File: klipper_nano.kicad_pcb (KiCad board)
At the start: 2 copper layers, 59.8 x 88.9 mm, 54 parts, among them J1 UART1, J10 ACC_PWR, J11 ACC_SPI, J2 PWR_IN, J3 TFT, J4 USB_A, J5 USB_A, J6 PWR_OUT, J7 USB_B_Mini, J8 UART2, J9 PWC, Q1 IRLML6344TRPBF, Q2 IRLML6402, U1 FT230XS, U2 PC817, U3 74HC04, U4 74HC4094, U5 74HC4094, U6 74HC4040, U7 ISO7721, U8 USBLC6-4SC6

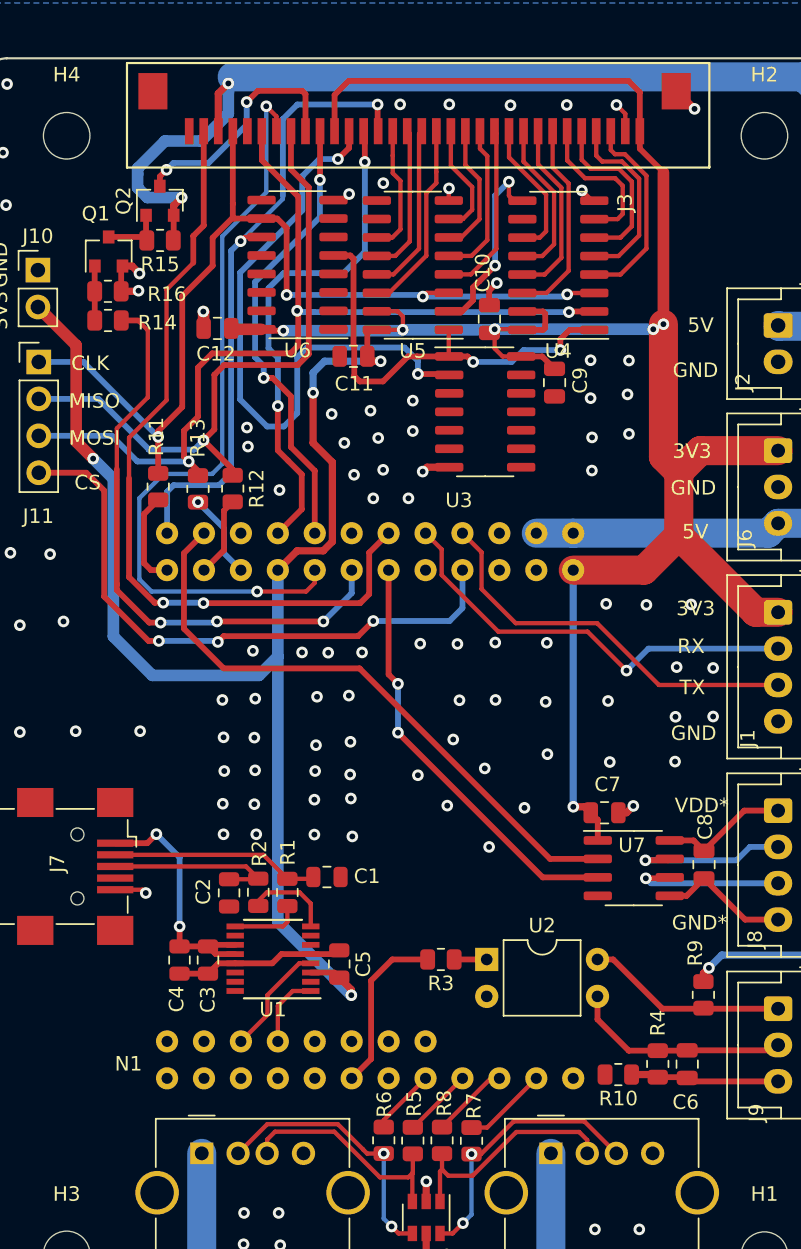
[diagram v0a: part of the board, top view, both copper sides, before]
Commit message: v2
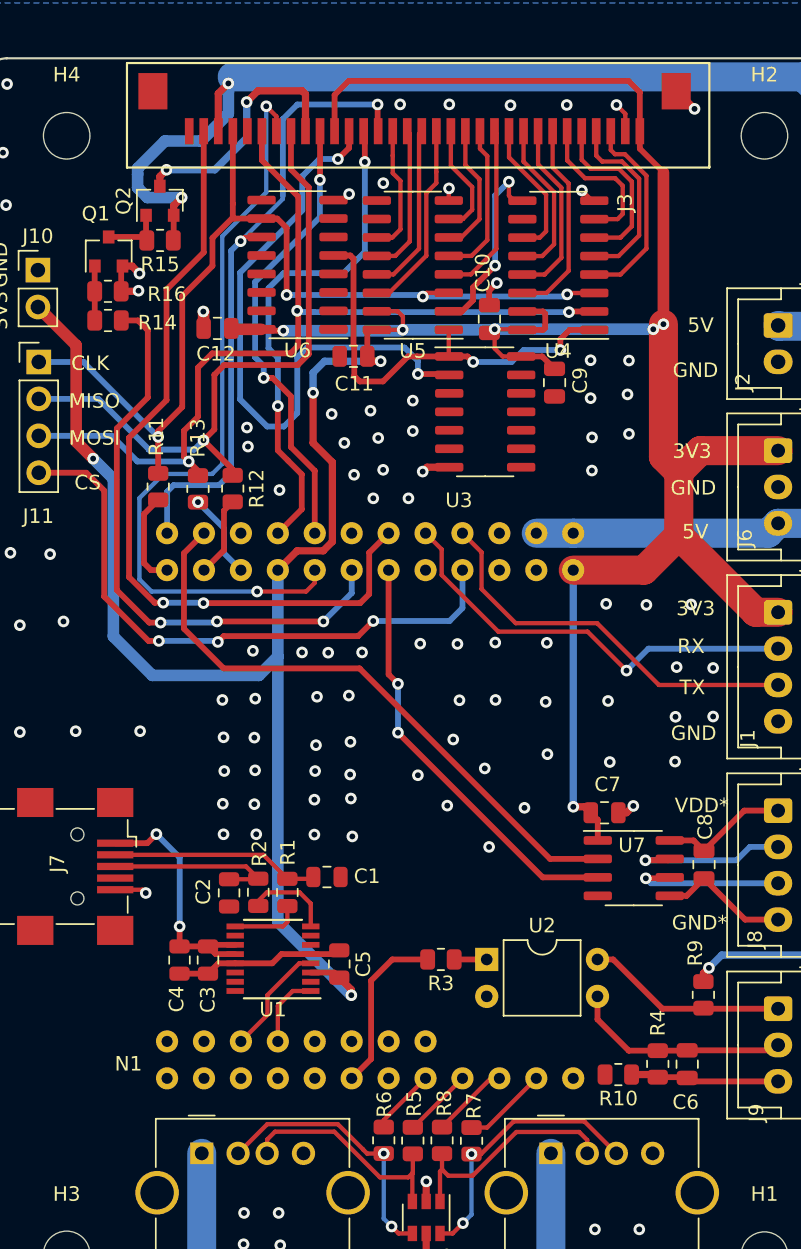
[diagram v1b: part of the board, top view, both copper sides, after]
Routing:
- net /16bit2SPI/TFT_LED: track 16.7 -> 17.2 mm
